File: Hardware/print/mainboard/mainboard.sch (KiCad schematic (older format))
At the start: 14 parts

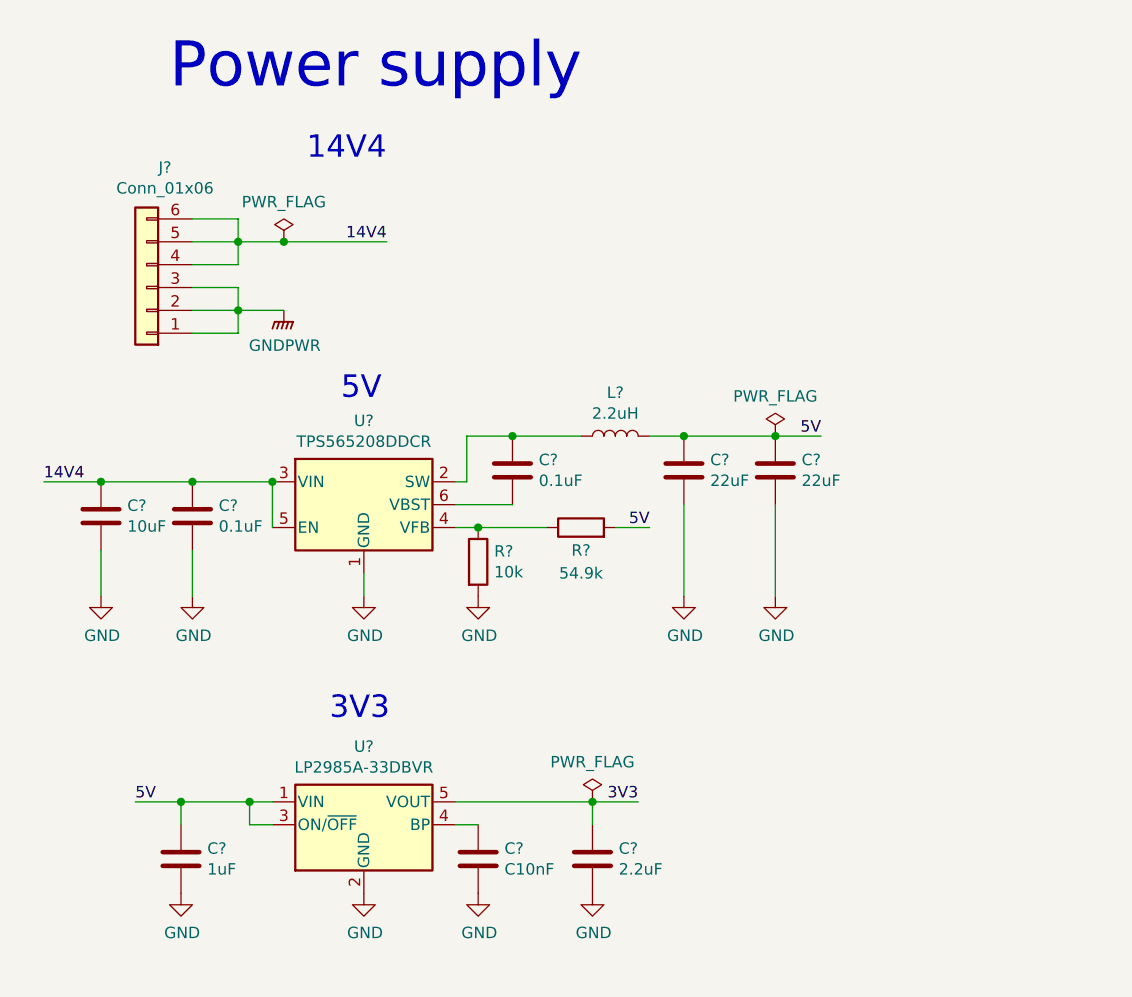
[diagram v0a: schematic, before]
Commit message: Speisung angepasst, ohne Stückliste
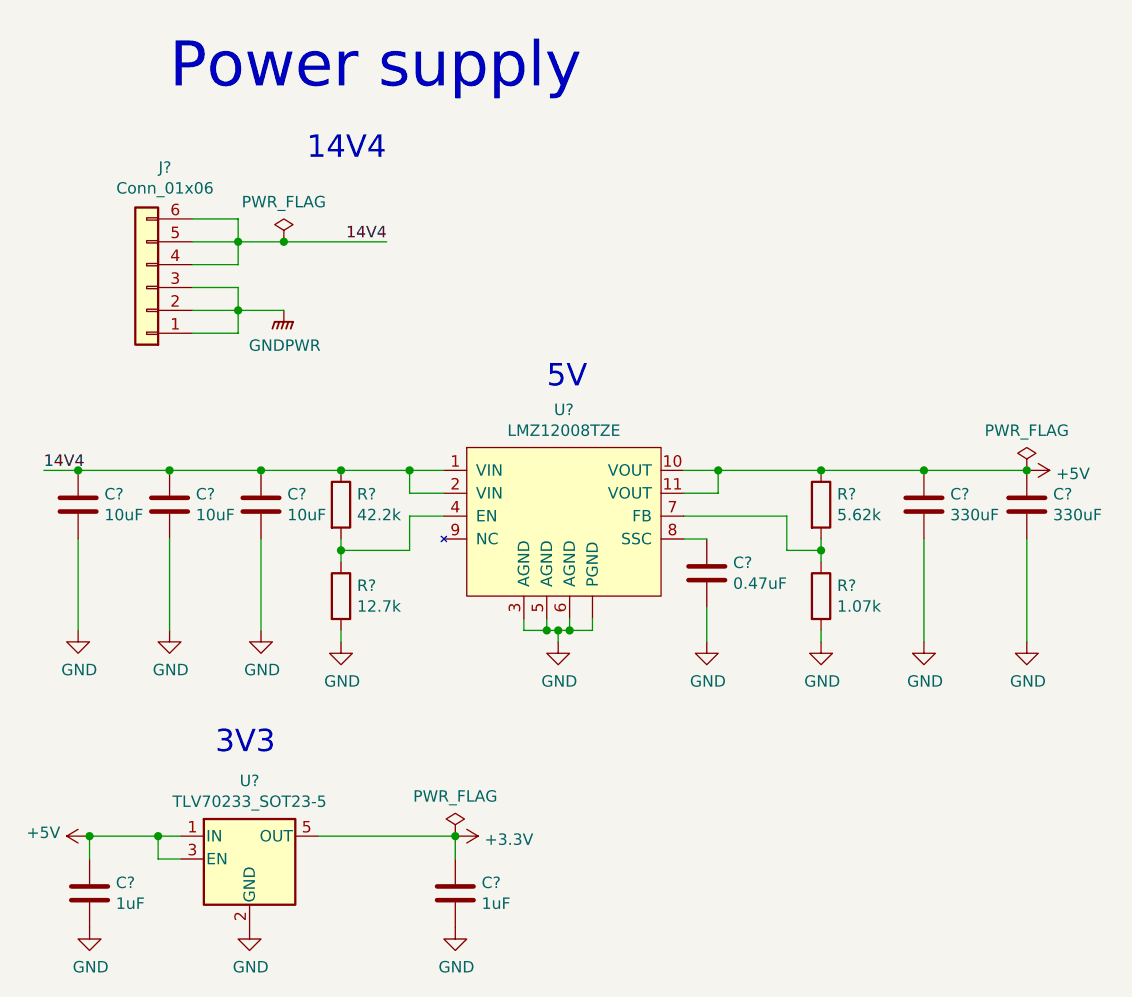
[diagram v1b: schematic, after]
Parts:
- removed C?: C10nF, symbol Device:C
- removed C?: 0.1uF, symbol Device:C
- removed C? (x2): 22uF, symbol Device:C
- removed L?: 2.2uH, symbol Device:L
- removed R?: 54.9k, symbol Device:R
- removed U?: LP2985A-33DBVR, Package_TO_SOT_SMD:SOT-23-5, symbol Regulator_Linear:LP2985-3.3
- removed U?: TPS565208DDCR, Package_TO_SOT_SMD:SOT-23-6, symbol Regulator_Switching:TPS562200
- added C? (x2): 10uF, symbol Device:C
- added C? (x2): 330uF, symbol Device:C
- added R?: 5.62k, symbol Device:R
- added R?: 42.2k, symbol Device:R
- added R?: 12.7k, symbol Device:R
- added U?: TLV70233_SOT23-5, Package_TO_SOT_SMD:SOT-23-5, symbol Regulator_Linear:TLV70233_SOT23-5
- added U?: LMZ12008TZE, symbol mylib:LMZ12008TZE
- C?: value 2.2uF -> 1uF
- C?: value 0.1uF -> 0.47uF
- R?: value 10k -> 1.07k
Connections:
- net 14V4: now also C?.1, C?.1, R?.1, U?.1 (VIN), U?.2 (VIN); no longer C?.1
- net GND: now also C?.2, C?.2, C?.2, C?.2, R?.2, U?.2 (GND), U?.3 (AGND), U?.5 (AGND), U?.6 (AGND), U?.~ (PGND)
- net at R?.1: now also R?.2, U?.7 (FB)
- net 3V3 renamed +3V3
- net +3V3: now also U?.5 (OUT)
- net 5V renamed +5V
- net +5V: now also C?.1, C?.1, R?.1, U?.1 (IN), U?.10 (VOUT), U?.11 (VOUT), U?.3 (EN)
- new net: C?.1, U?.8 (SSC)
- new net: R?.1, R?.2, U?.4 (EN)
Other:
- moved on the sheet: C?, R?
